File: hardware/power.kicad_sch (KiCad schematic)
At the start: 12 parts

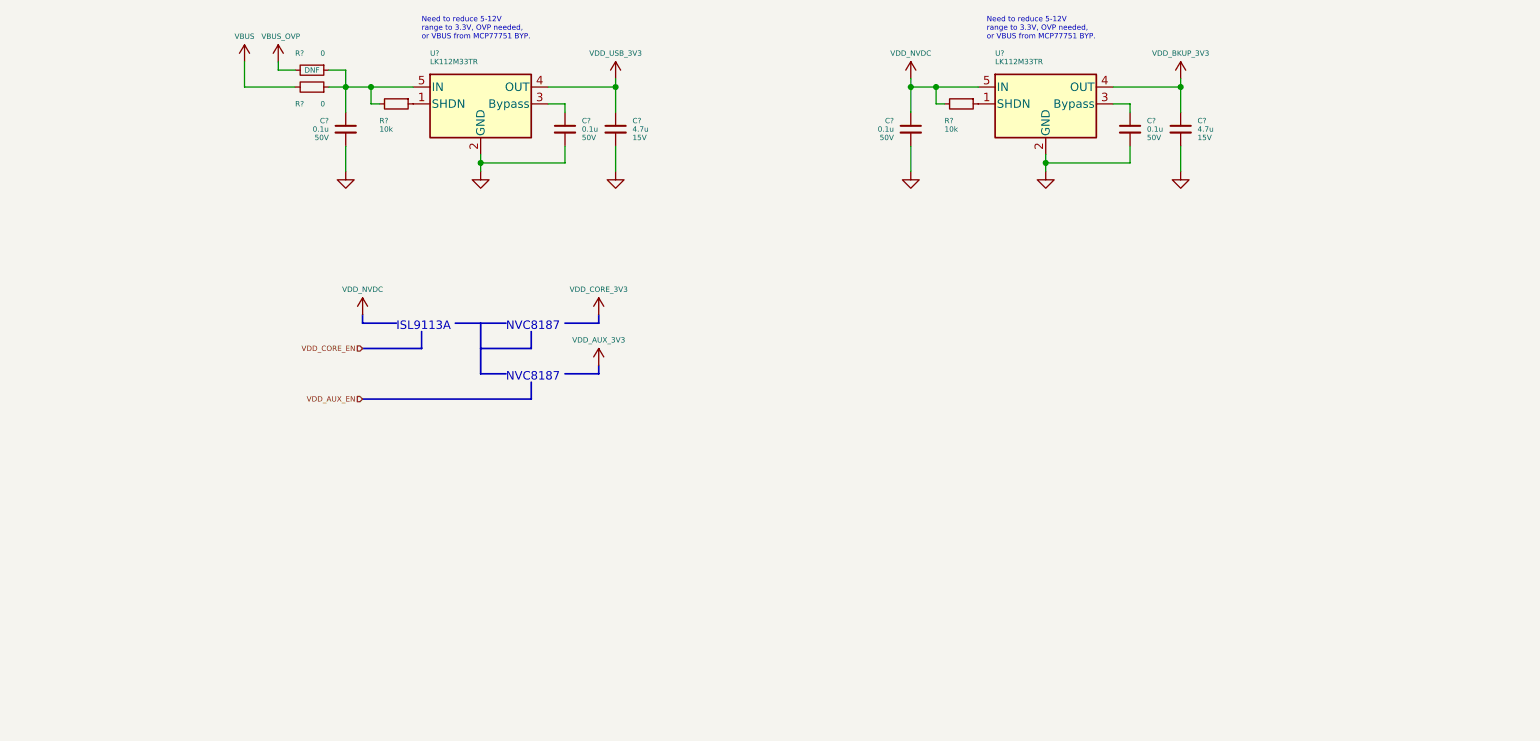
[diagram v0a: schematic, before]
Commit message: ready for first review
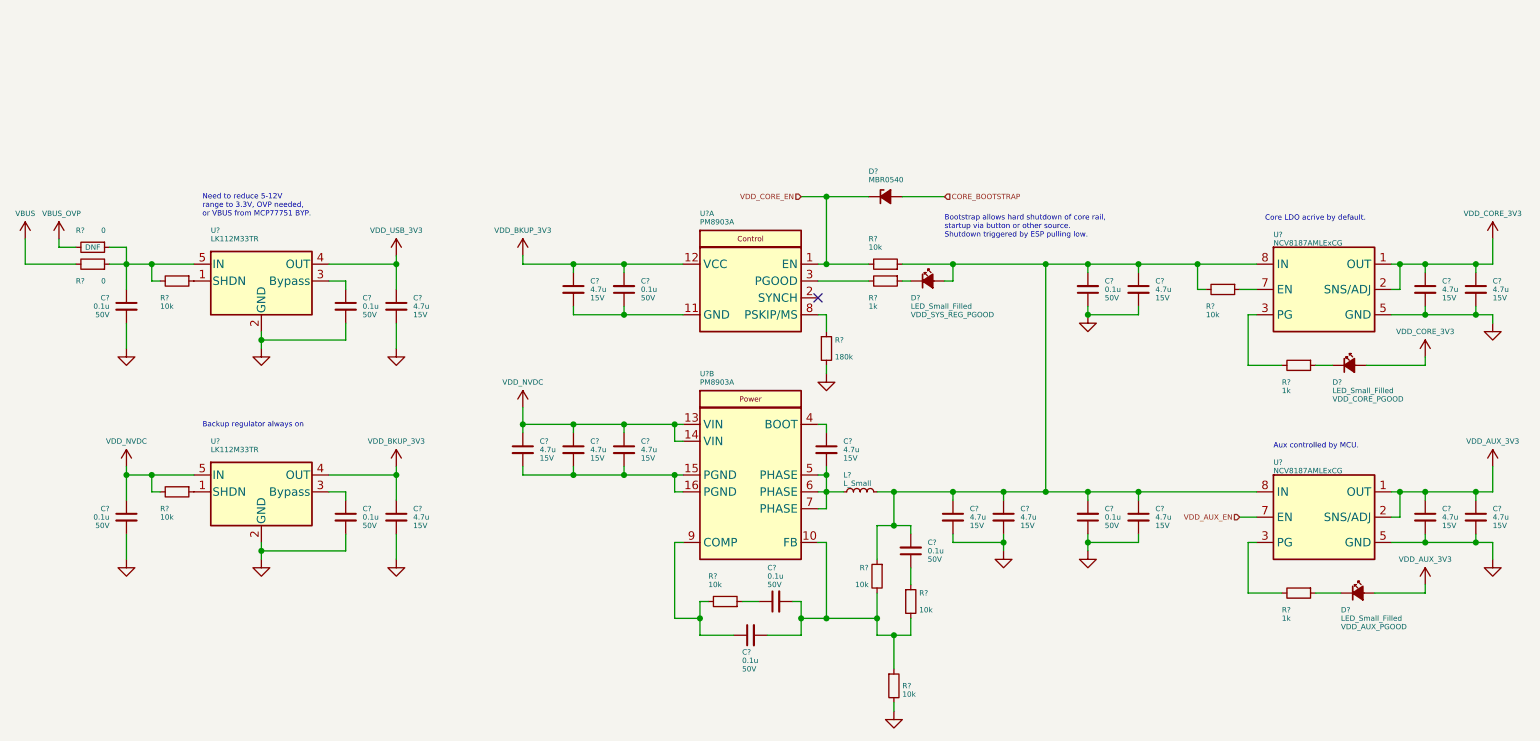
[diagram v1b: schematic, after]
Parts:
- added C? (x6): 0.1u, Capacitor_SMD:C_0603_1608Metric, symbol Device:C_Small
- added C? (x13): 4.7u, Capacitor_SMD:C_0603_1608Metric, symbol Device:C_Small
- added D?: MBR0540, symbol Device:D_Zener_Small_Filled
- added D? (x3): LED_Small_Filled, symbol Device:LED_Small_Filled
- added L?: L_Small, symbol Device:L_Small
- added R? (x3): 1k, Resistor_SMD:R_0603_1608Metric, symbol Device:R_Small
- added R? (x6): 10k, Resistor_SMD:R_0603_1608Metric, symbol Device:R_Small
- added R?: 180k, Resistor_SMD:R_0603_1608Metric, symbol Device:R_Small
- added U? (x2): NCV8187AMLExCG, Package_DFN_QFN:DFN-8-1EP_3x3mm_P0.65mm_EP1.55x2.4mm, symbol bt_PMIC_Linear:NCV8187AMLExCG
- added U? (x2): PM8903A, Package_DFN_QFN:VQFN-16-1EP_3x3mm_P0.5mm_EP1.45x1.45mm_ThermalVias, symbol bt_PMIC_DCDC_Buck:PM8903A
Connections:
- net 3V3_CORE: now also C?.1, C?.1, D?.2 (A), U?.1 (OUT), U?.2 (SNS/ADJ)
- net GND: now also C?.1, C?.1, C?.2, C?.2, C?.2, C?.2, C?.2, C?.2, C?.2, C?.2, R?.2, R?.2, U?.5 (GND), U?.5 (GND), U?.9 (GND), U?.9 (GND)
- net VCC_BKUP_3V3: now also C?.1, C?.2, U?.12 (VCC)
- net VDD_AUX_3V3: now also C?.1, C?.1, D?.2 (A), U?.1 (OUT), U?.2 (SNS/ADJ)
- net VDD_AUX_EN: now also U?.7 (EN)
- net VDD_CORE_EN: now also D?.1 (K), R?.2, U?.1 (EN)
- net VDD_NVDC: now also C?.1, C?.1, C?.1, U?.13 (VIN), U?.14 (VIN)
- new net: D?.1 (K), R?.1 (x3)
- new net: R?.2, U?.3 (PG) (x2)
- new net: C?.1, C?.2, U?.11 (GND)
- new net: C?.1, R?.1 (x2)
- new net: C?.2, C?.2, R?.1, R?.2, R?.2, U?.10 (FB)
- new net: C?.1, C?.1, C?.1, C?.1, C?.2, C?.2, C?.2, D?.2 (A), L?.2, R?.1, R?.1, R?.2, U?.8 (IN), U?.8 (IN)
- new net: R?.1, U?.7 (EN)
- new net: R?.1, U?.8 (PSKIP/MS)
- new net: C?.1, R?.2, U?.9 (COMP)
- new net: C?.2, L?.1, U?.5 (PHASE), U?.6 (PHASE), U?.7 (PHASE)
- new net: C?.1, U?.4 (BOOT)
- new net: C?.2, C?.2, C?.2, U?.15 (PGND), U?.16 (PGND)
- new net: R?.2, U?.3 (PGOOD)
- new net CORE_BOOTSTRAP: D?.2 (A)
- no-connect marks 0 -> 1
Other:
- note added: "Aux controlled by MCU."
- note added: "Backup regulator always on"
- note added: "Bootstrap allows hard shutdown of core rail, startup via button or other source. Shutdown triggered by ESP pulling low."
- note added: "Core LDO acrive by default."
- note removed: "ISL9113A"
- note removed: "NVC8187"
- moved on the sheet: C?, R?, U?
